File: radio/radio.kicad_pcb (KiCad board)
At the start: 2 copper layers, 27.7 x 15.1 mm, 18 parts, among them J1 Conn_02x04_Top_Bottom, U1 NRF24L01, Y1 16mhz

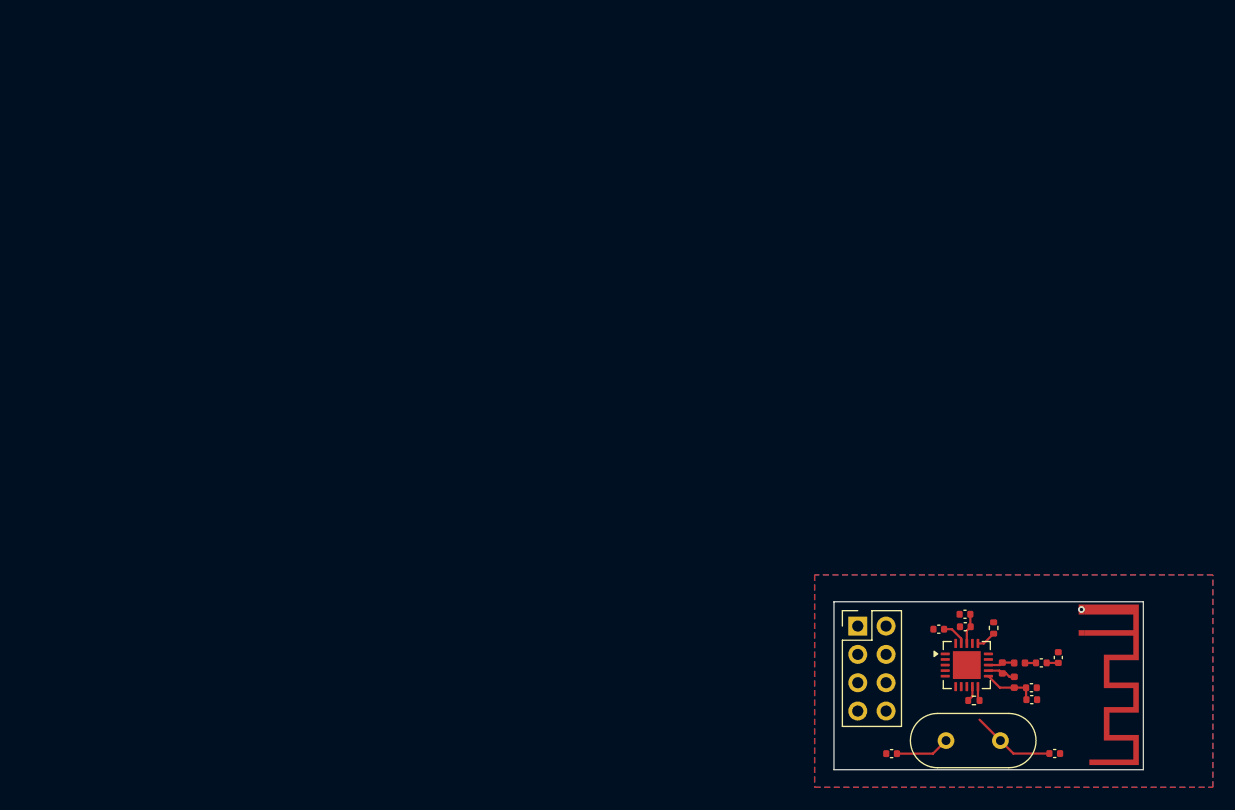
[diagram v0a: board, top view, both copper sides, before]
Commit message: Update Readme
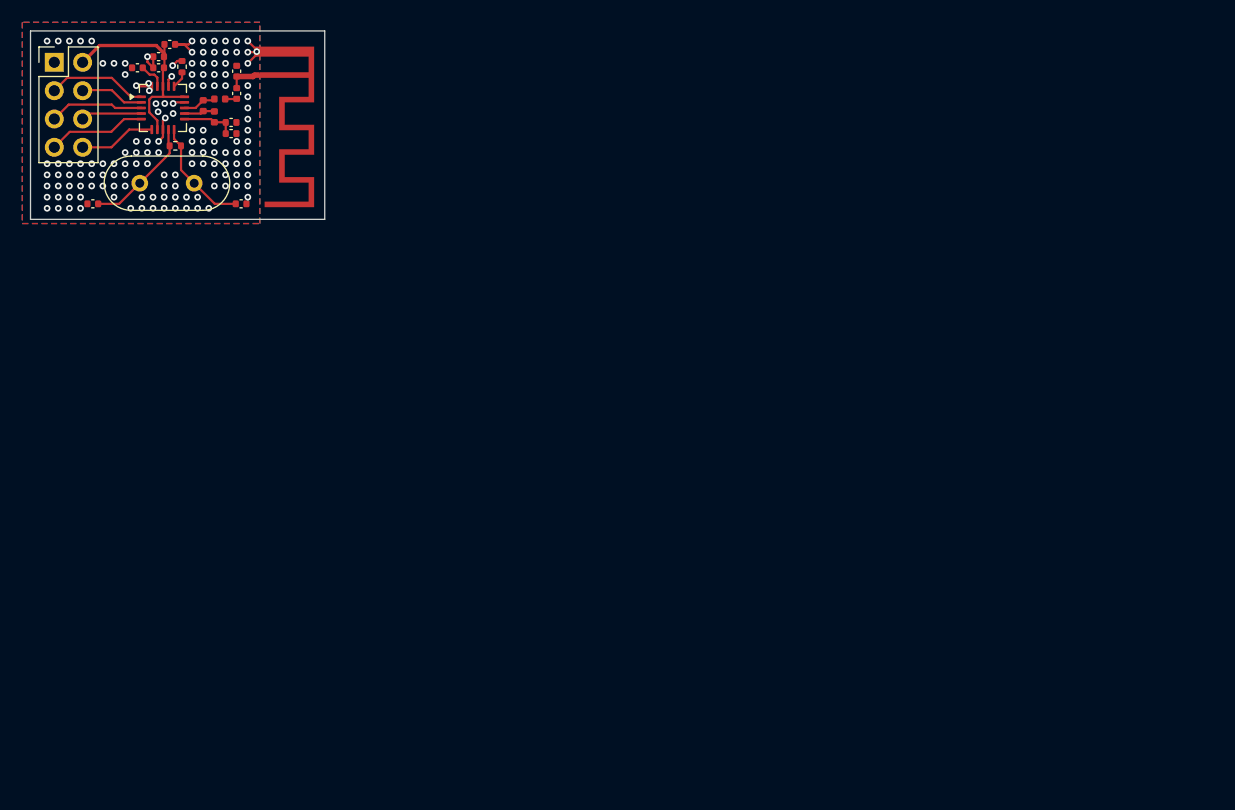
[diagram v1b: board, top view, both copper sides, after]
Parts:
- removed the C7 at (115.9, 78.7)
- removed the C9 at (118.3, 77.3)
- removed the R2 at (120.8, 78.6)
- added C1: 4.7uF, Capacitor_SMD:C_0402_1005Metric, F.Cu at (46.9, 26.2)
- added C2: 10nF, Capacitor_SMD:C_0402_1005Metric, F.Cu at (45.9, 28.3)
- added C3: 1nF, Capacitor_SMD:C_0402_1005Metric, F.Cu at (45.9, 27.3)
- added R1: 22K, Resistor_SMD:R_0402_1005Metric, F.Cu at (48.0, 28.2)
- C8: value 1nF -> 33nF
- moved C7 90.5 mm to (52.9, 28.6)
- moved C8 89.6 mm to (44.0, 28.3)
- moved AE1 89.3 mm to (56.8, 33.9)
- moved C6 88.4 mm to (52.9, 30.6), turned to 90 degrees
- moved C9 88.1 mm to (53.3, 40.5)
- moved J1 88.0 mm to (36.6, 27.9)
- moved C5 87.9 mm to (52.4, 34.2)
- moved Y1 87.9 mm to (44.3, 38.7)
- moved C4 87.9 mm to (52.4, 33.2)
- moved L1 87.8 mm to (50.9, 32.7)
- moved L3 87.8 mm to (51.4, 31.1)
- moved U1 87.7 mm to (46.3, 31.9)
- moved L2 87.6 mm to (49.9, 31.7)
- moved R2 87.2 mm to (47.4, 35.3)
- moved C10 87.0 mm to (40.0, 40.5)
- renumbered C2 to C10, C3 to C4, C4 to C5, C5 to C6, C6 to C7, C1 to C9, L2 to L1, L1 to L2, R1 to R2
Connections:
- C8 pad 1: VDD -> Net-(U1-DVDD)
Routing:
- net GND: track 0.00 -> 17.3 mm, vias 1 -> 140
- net VDD: track 2.77 -> 19.5 mm
- net CE: track 0.00 -> 8.99 mm
- net MISO: track 0.00 -> 8.85 mm
- net SCK: track 0.00 -> 8.46 mm
- net IRQ: track 0.00 -> 6.86 mm
- net CSN: track 0.00 -> 5.74 mm
- net MOSI: track 0.00 -> 5.47 mm
- net XC2: track 6.28 -> 10.5 mm
- net Net-(AE1-PCB_Trace): track 1.04 -> 2.69 mm
- net XC1: track 8.81 -> 10.1 mm
- net Net-(U1-ANT2): track 2.42 -> 3.01 mm
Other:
- board size 27.7 x 15.1 mm -> 26.4 x 16.9 mm
